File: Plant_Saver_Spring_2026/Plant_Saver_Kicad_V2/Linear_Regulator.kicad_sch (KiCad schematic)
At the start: 7 parts, among them U12 LP38511TJ-ADJ/NOPB

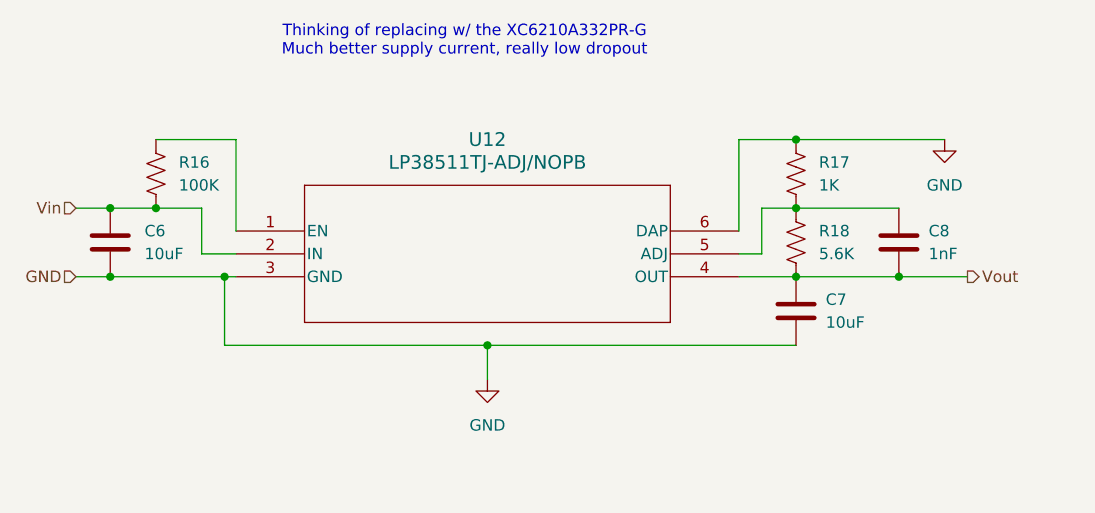
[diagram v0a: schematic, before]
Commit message: Organized Repo
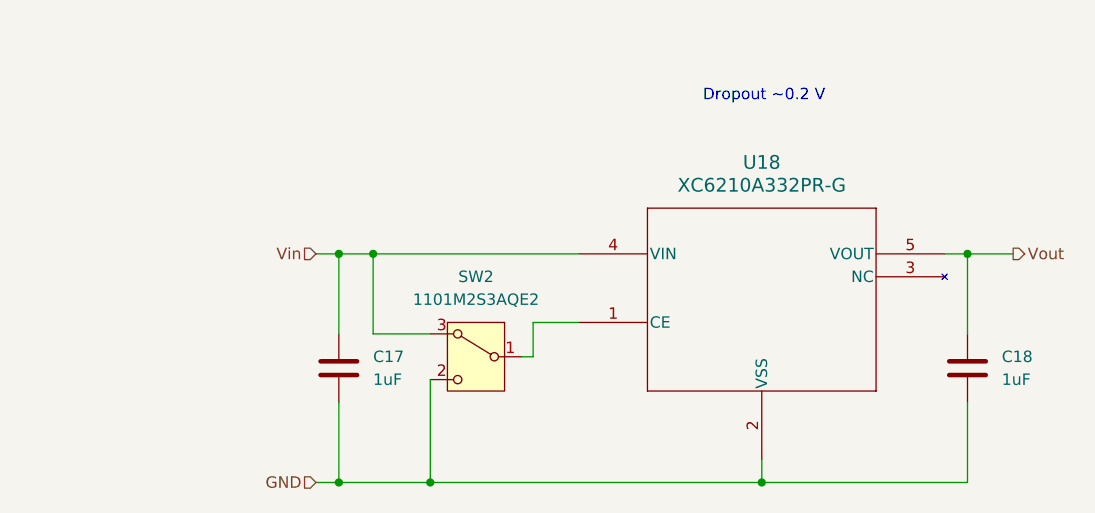
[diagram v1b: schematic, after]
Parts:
- removed C6, C7: 10uF, Capacitor_SMD:C_1206_3216Metric_Pad1.33x1.80mm_HandSolder, symbol Device:C
- removed C8: 1nF, Capacitor_SMD:C_1206_3216Metric_Pad1.33x1.80mm_HandSolder, symbol Device:C
- removed R16: 100K, Resistor_SMD:R_1206_3216Metric_Pad1.30x1.75mm_HandSolder, symbol Device:R_US
- removed R17: 1K, Resistor_THT:R_Axial_DIN0207_L6.3mm_D2.5mm_P10.16mm_Horizontal, symbol Device:R_US
- removed R18: 5.6K, Resistor_THT:R_Axial_DIN0207_L6.3mm_D2.5mm_P10.16mm_Horizontal, symbol Device:R_US
- removed U12: LP38511TJ-ADJ/NOPB, LP38511TJ_ADJ_NOPB:TJ5A_TEX, symbol LP38511TJ_ADJ_NOPB:LP38511TJ-ADJ_NOPB
- added C17, C18: 1uF, Capacitor_SMD:C_1206_3216Metric_Pad1.33x1.80mm_HandSolder, symbol Device:C
- added SW2: 1101M2S3AQE2, 1101M2S3AQE2:SPDT-1101M2_CNK, symbol Switch:SW_Wuerth_450301014042
- added U18: XC6210A332PR-G, Package_TO_SOT_SMD:SOT-89-5_Handsoldering, symbol XC6210A332PR-G:XC6210A332PR-G
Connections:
- net GND: now also C17.2, C18.2, SW2.2 (C), U18.2 (VSS)
- net Vin: now also C17.1, SW2.3 (A), U18.4 (VIN)
- net Vout: now also C18.1, U18.5 (VOUT)
- new net: SW2.1 (B), U18.1 (CE)
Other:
- note added: "Dropout ~0.2 V"
- note removed: "Thinking of replacing w/ the XC6210A332PR-G Much better supply current, really low dropout"
